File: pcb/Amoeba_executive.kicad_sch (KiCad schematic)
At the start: 4 parts, among them J1 Conn_01x04_MountingPin, J2 Conn_01x04_MountingPin, SW1 SW_PUSH_LED

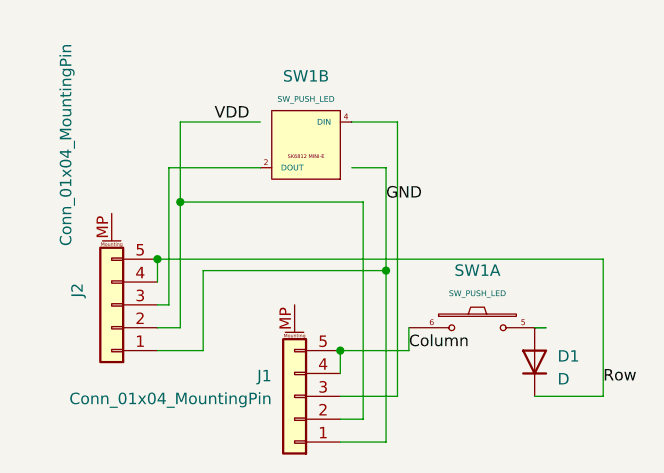
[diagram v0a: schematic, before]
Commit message: First draft complete
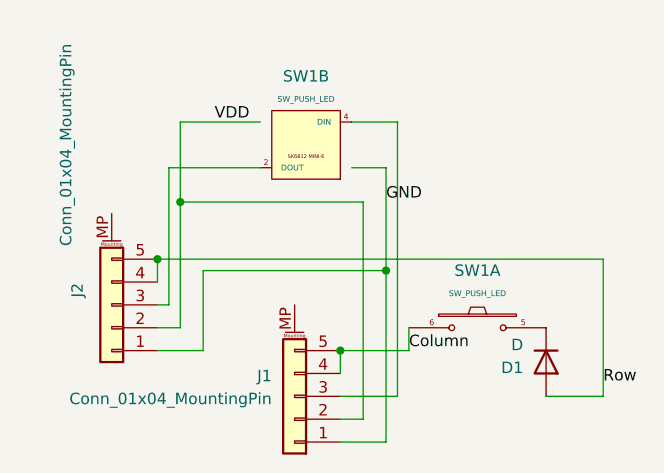
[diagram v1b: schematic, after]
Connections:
- net Row: now also D1.2 (A); no longer D1.1 (K)
- net at SW1.5: now also D1.1 (K); no longer D1.2 (A)
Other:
- moved on the sheet: D1
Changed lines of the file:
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@@
     (stroke (width 0) (type default))
   )
-  (wire (pts (xy 149.86 72.39) (xy 157.48 72.39))
+  (wire (pts (xy 151.13 72.39) (xy 157.48 72.39))
     (stroke (width 0) (type default))
   )
@@
   )
   (wire (pts (xy 110.49 41.91) (xy 119.38 41.91))
-    (stroke (width 0) (type default))
-  )
-  (wire (pts (xy 151.13 64.77) (xy 149.86 64.77))
     (stroke (width 0) (type default))
   )
@@
     )
   )
-  (symbol (lib_id "Device:D") (at 149.86 68.58 90) (unit 1)
+  (symbol (lib_id "Device:D") (at 151.13 68.58 270) (unit 1)
     (in_bom yes) (on_board yes) (dnp no)
-    (property "Reference" "D1" (at 152.4 67.945 90)
+    (property "Reference" "D1" (at 148.59 69.215 90)
       (effects (font (size 1.27 1.27)) (justify right))
     )
-    (property "Value" "D" (at 152.4 70.485 90)
+    (property "Value" "D" (at 148.59 66.675 90)
       (effects (font (size 1.27 1.27)) (justify right))
     )
-    (property "Footprint" "ergodonk_kicad_library:D_SOD-123_DO-35_Hybrid_DoubleSided" (at 149.86 68.58 0)
+    (property "Footprint" "ergodonk_kicad_library:D_SOD-123_DO-35_Hybrid_DoubleSided" (at 151.13 68.58 0)
       (effects (font (size 1.27 1.27)) hide)
     )
-    (property "Datasheet" "~" (at 149.86 68.58 0)
+    (property "Datasheet" "~" (at 151.13 68.58 0)
       (effects (font (size 1.27 1.27)) hide)
     )
-    (property "Sim.Device" "D" (at 149.86 68.58 0)
+    (property "Sim.Device" "D" (at 151.13 68.58 0)
       (effects (font (size 1.27 1.27)) hide)
     )
-    (property "Sim.Pins" "1=K 2=A" (at 149.86 68.58 0)
+    (property "Sim.Pins" "1=K 2=A" (at 151.13 68.58 0)
       (effects (font (size 1.27 1.27)) hide)
     )
